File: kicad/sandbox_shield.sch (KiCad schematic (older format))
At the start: 7 parts

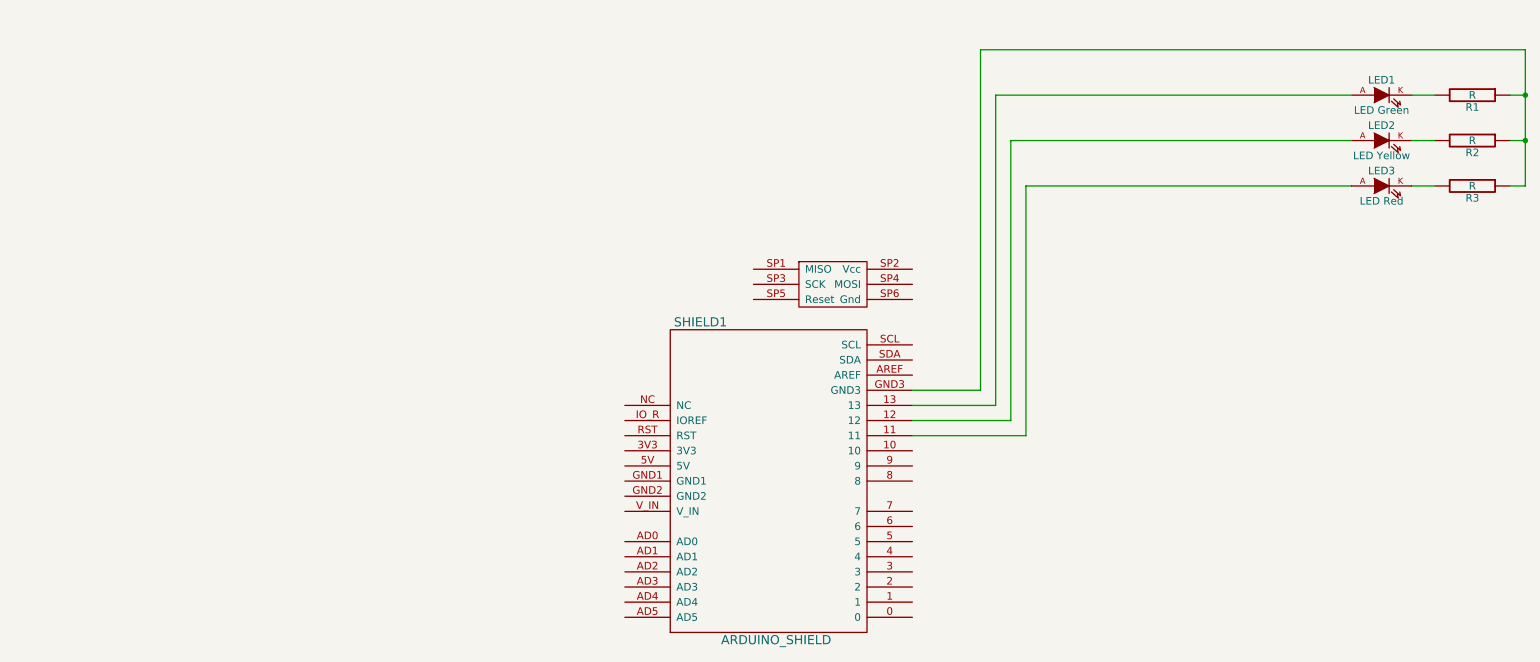
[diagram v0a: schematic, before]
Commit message: Engadido o LDR Algún cambio na documentación
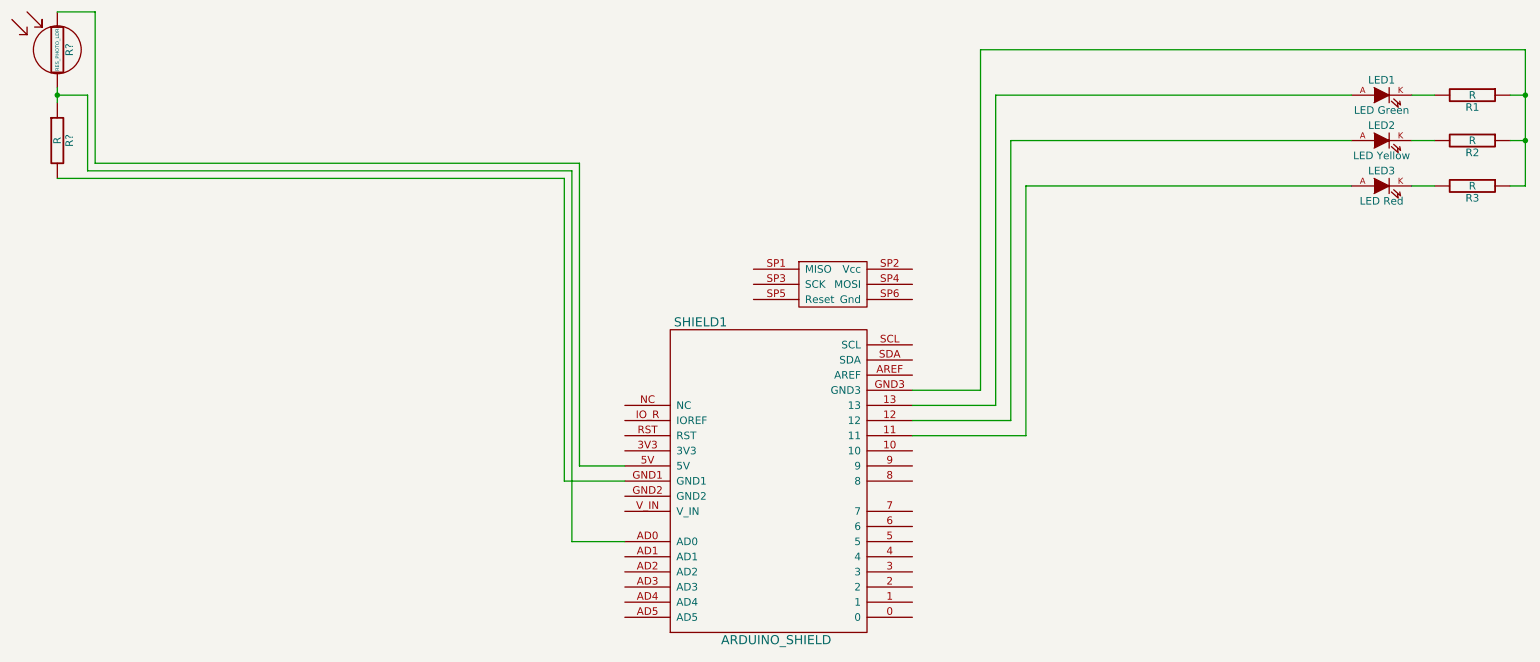
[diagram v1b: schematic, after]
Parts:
- added R?: RES_PHOTO_LDR, symbol RES_PHOTO_LDR
- added R?: R, symbol R
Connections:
- net at SHIELD1.5V: now also R?.1
- net at SHIELD1.AD0: now also R?.1, R?.2
- net at SHIELD1.GND1: now also R?.2
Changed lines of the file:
@@
 	7400 3550 7400 1900
 Wire Wire Line
-	10600 1900 10700 1900
+	10700 1900 10600 1900
 Wire Wire Line
-	10700 1900 10700 1000
+	10700 1000 10700 1900
 Wire Wire Line
 	10700 1000 7100 1000
@@
 	10600 1300 10700 1300
 Connection ~ 10700 1300
+$Comp
+L RES_PHOTO_LDR R?
+U 1 1 55875939
+P 1000 1000
+F 0 "R?" V 1080 1000 50  0000 C CNN
+F 1 "RES_PHOTO_LDR" V 1000 1000 24  0000 C CNN
+F 2 "" H 1000 1000 60  0000 C CNN
+F 3 "" H 1000 1000 60  0000 C CNN
+	1    1000 1000
+	1    0    0    -1
+$EndComp
+$Comp
+L R R?
+U 1 1 55875B0A
+P 1000 1600
+F 0 "R?" V 1080 1600 50  0000 C CNN
+F 1 "R" V 1000 1600 50  0000 C CNN
+F 2 "" H 1000 1600 60  0000 C CNN
+F 3 "" H 1000 1600 60  0000 C CNN
+	1    1000 1600
+	1    0    0    -1
+$EndComp
+Wire Wire Line
+	1000 1250 1000 1350
+Connection ~ 1000 1300
+Wire Wire Line
+	1200 1300 1000 1300
+Wire Wire Line
+	1000 1850 4350 1850
+Wire Wire Line
+	4350 1850 4350 3850
+Wire Wire Line
+	4350 3850 4750 3850
+Wire Wire Line
+	1200 1300 1200 1800
+Wire Wire Line
+	1200 1800 4400 1800
+Wire Wire Line
+	4400 1800 4400 4250
+Wire Wire Line
+	4400 4250 4750 4250
+Wire Wire Line
+	1000 750  1250 750
+Wire Wire Line
+	1250 750  1250 1750
+Wire Wire Line
+	1250 1750 4450 1750
+Wire Wire Line
+	4450 1750 4450 3750
+Wire Wire Line
+	4450 3750 4750 3750
 $EndSCHEMATC
